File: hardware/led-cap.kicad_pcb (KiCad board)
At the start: 2 copper layers, 76.2 x 50.8 mm, 10 parts, among them IC1 ATTINY20-X, K1 CONN_3, P1 CONN_2, P2 CONN_6, Q1 IRLML2402PbF, U1 MMA7660

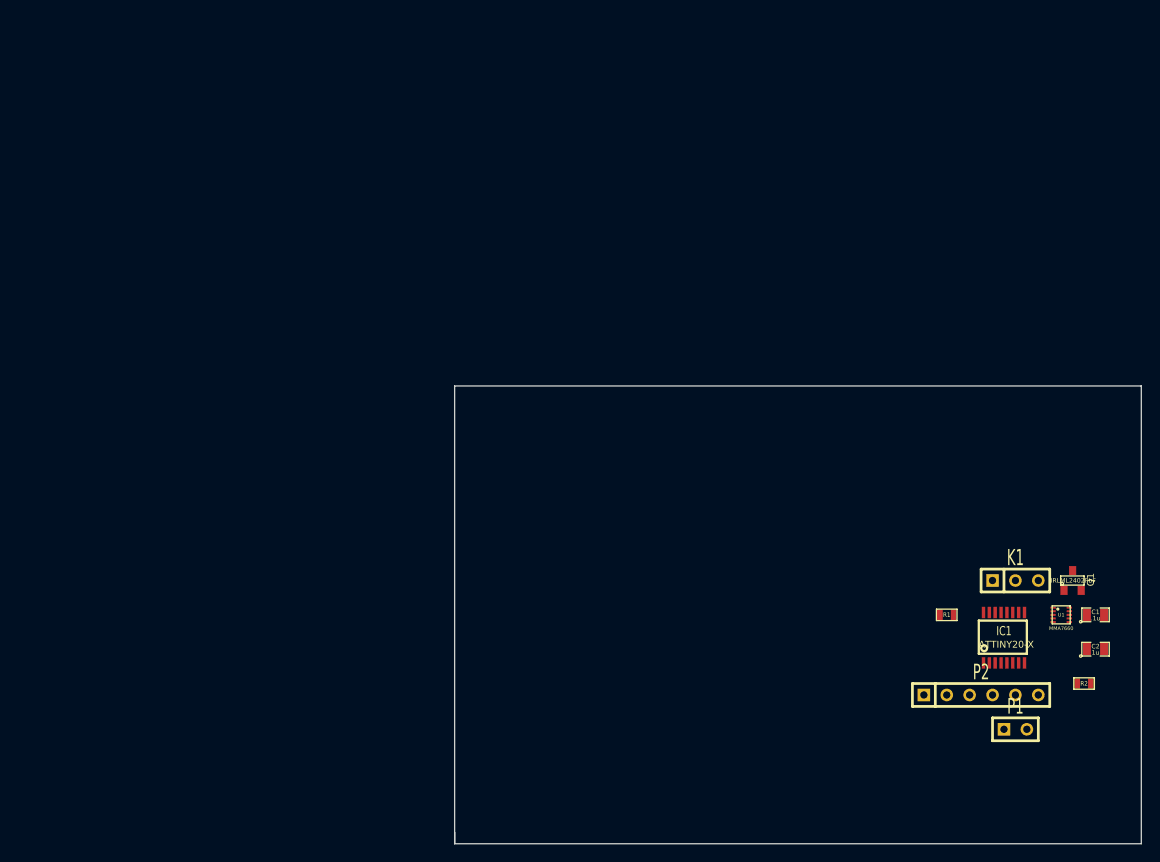
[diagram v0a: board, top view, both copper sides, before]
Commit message: Cleanup and PCB Layout
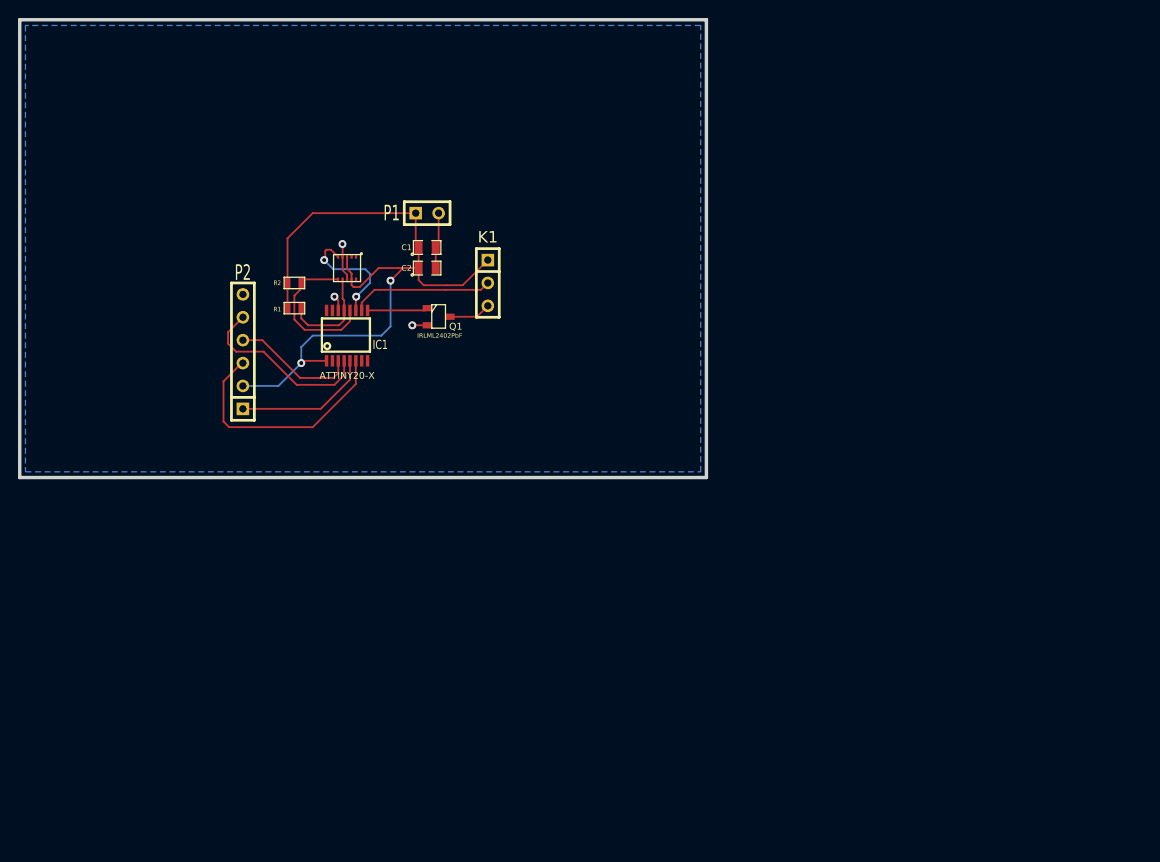
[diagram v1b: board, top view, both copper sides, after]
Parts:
- C1, C2: footprint SMD_Packages:SM0805 -> SM0805
- IC1: footprint SMD_Packages:TSSOP16 -> TSSOP16
- K1: footprint Connect:SIL-3 -> SIL-3
- P1: footprint Connect:SIL-2 -> SIL-2
- P2: footprint Connect:SIL-6 -> SIL-6
- Q1: footprint SMD_Packages:SOT23 -> SOT23
- R1, R2: footprint SMD_Packages:SM0603 -> SM0603
- U1: footprint tom:DFN-10 -> DFN10
- moved R2 98.3 mm to (61.0, 71.1)
- moved P2 90.3 mm to (55.2, 78.7), turned to 90 degrees
- moved U1 88.1 mm to (66.8, 69.5), turned to 180 degrees
- moved P1 86.8 mm to (75.7, 63.4)
- moved C2 85.4 mm to (75.7, 69.5)
- moved C1 84.6 mm to (75.7, 67.2)
- moved IC1 80.2 mm to (66.8, 77.0)
- moved R1 80.0 mm to (61.0, 73.9)
- moved Q1 76.2 mm to (77.0, 74.9), turned to 270 degrees
- moved K1 67.2 mm to (82.4, 71.1), turned to 270 degrees
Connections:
- IC1 pad 2: Net-(IC1-Pad2) -> (no net)
- IC1 pad 7: Net-(IC1-Pad7) -> (no net)
- IC1 pad 8: Net-(IC1-Pad8) -> (no net)
- U1 pad 1: Net-(U1-Pad1) -> (no net)
- U1 pad 10: Net-(U1-Pad10) -> (no net)
- U1 pad 2: Net-(U1-Pad2) -> (no net)
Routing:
- net VCC: track 0.00 -> 83.4 mm, vias 0 -> 2
- net N-000011: track 0.00 -> 27.0 mm
- net N-000007: track 0.00 -> 20.4 mm
- net N-000010: track 0.00 -> 16.9 mm
- net N-000002: track 0.00 -> 15.8 mm
- net N-000014: track 0.00 -> 15.3 mm
- net N-000006: track 0.00 -> 13.9 mm
- net GND: track 0.00 -> 13.7 mm, vias 0 -> 3
- net N-000001: track 0.00 -> 13.3 mm, vias 0 -> 2
- net N-000009: track 0.00 -> 11.1 mm
- net N-000004: track 0.00 -> 6.72 mm
- net N-000003: track 0.00 -> 4.69 mm
- added copper zone on B.Cu, net GND
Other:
- outline, holes or cut-outs redrawn
- net class Default: trace_width 0.254 -> 0.2032
- rule pad_to_mask_clearance: 0 -> 0.254
- rule trace_min: 0.254 -> 0.2032
